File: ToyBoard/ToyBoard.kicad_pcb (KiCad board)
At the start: 2 copper layers, 41.3 x 41 mm, 18 parts, among them J5 MSD-1-A, Q1 NMOS, Q2 NMOS

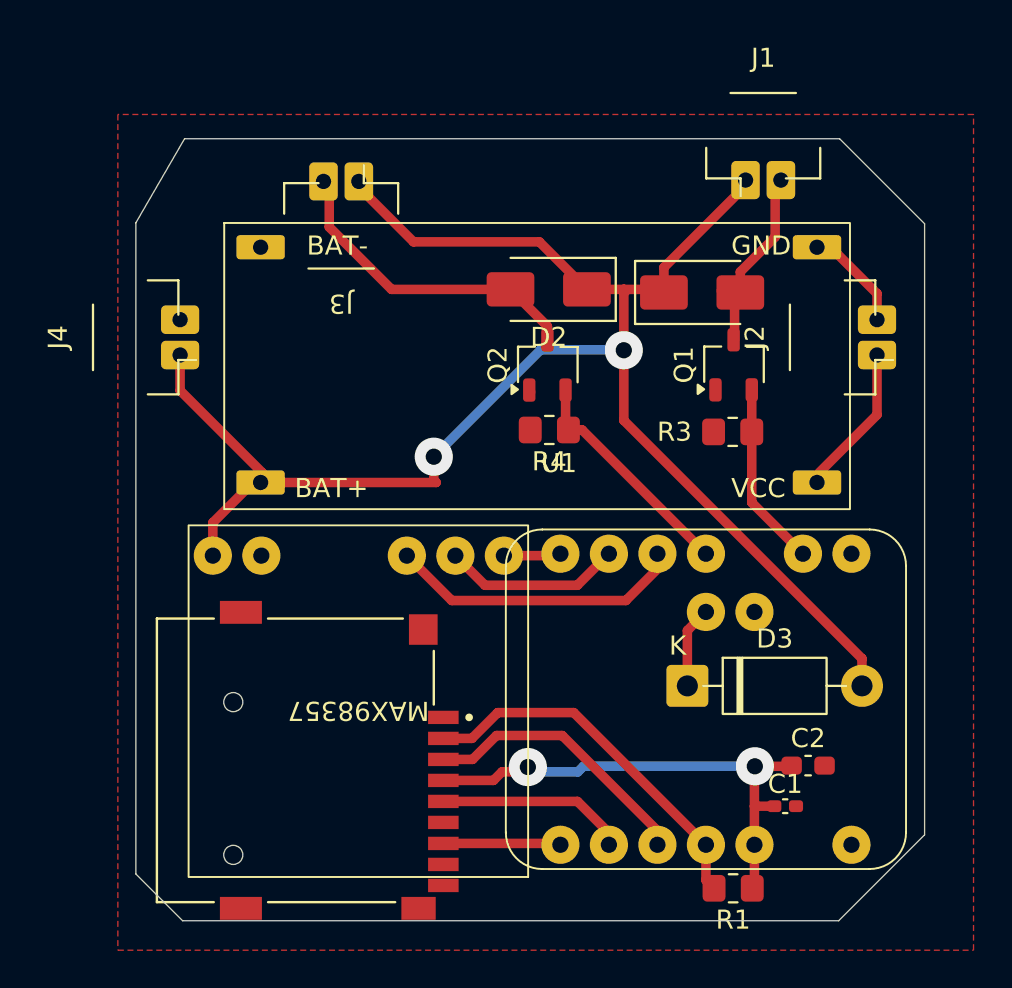
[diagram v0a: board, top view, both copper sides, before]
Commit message: Pcb and Gerbs for JLCPCB
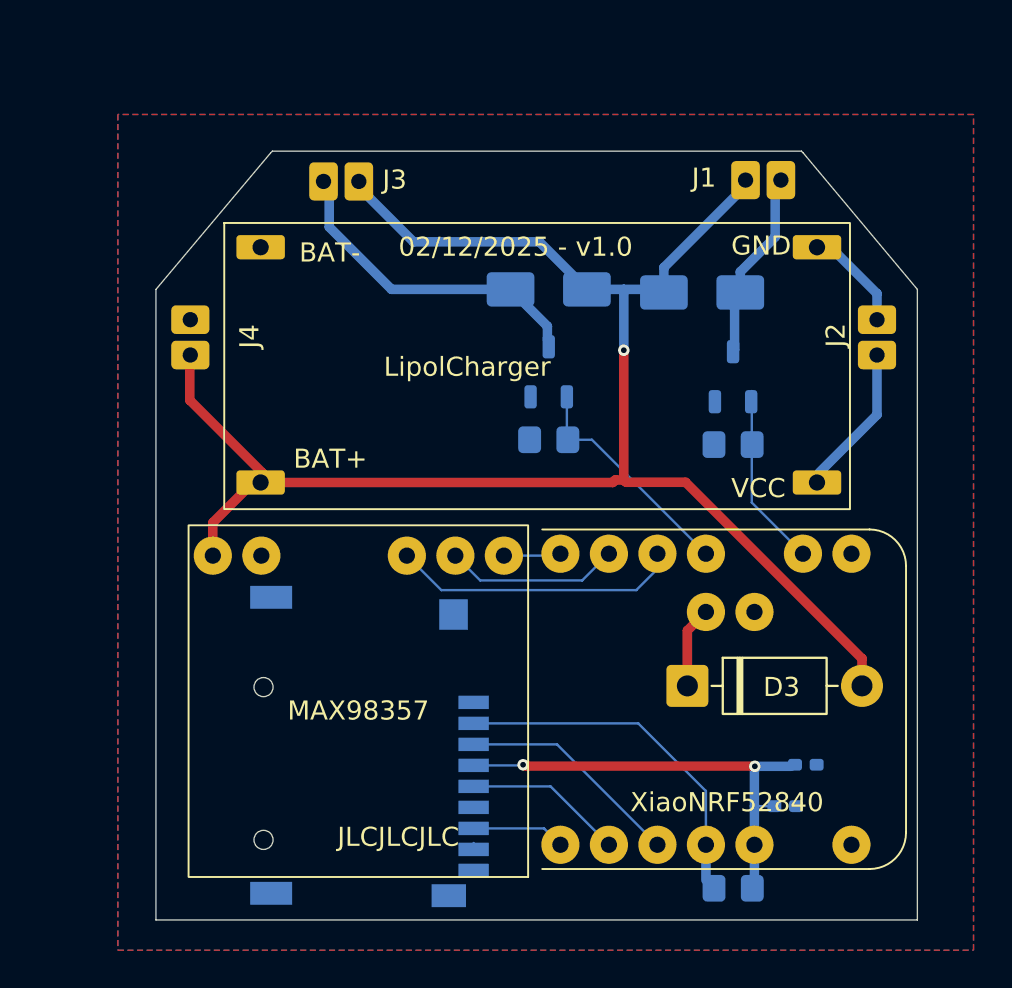
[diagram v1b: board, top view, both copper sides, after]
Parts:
- C1, D1, D2, J5, Q1, Q2, R1, R3, R4: moved to B.Cu
- C2: footprint Capacitor_SMD:C_0603_1608Metric_Pad1.08x0.95mm_HandSolder -> Capacitor_SMD:C_0402_1005Metric_Pad0.74x0.62mm_HandSolder; moved to B.Cu
- moved J5 1.77 mm to (126.0, 124.7), turned to 90 degrees
- moved R3 0.67 mm to (147.3, 109.0)
- moved Q1 0.62 mm to (147.3, 105.4)
- moved J4 0.54 mm to (117.6, 103.3)
- moved R4 0.51 mm to (137.7, 108.7)
- moved Q2 0.36 mm to (137.7, 105.2)
- moved C2 0.13 mm to (151.1, 125.7)
- renumbered U1 to LipolCharger, XiaoNRF1 to XiaoNRF52840
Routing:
- net BAT+: track 89.0 -> 86.3 mm, vias 2 -> 1
- net Net-(J5-VDD): track 26.3 -> 24.0 mm
- net Net-(J5-CMD): track 14.5 -> 12.5 mm
- net Net-(J5-CD/DAT3): track 19.6 -> 18.3 mm
- net Net-(J5-DAT0): track 6.16 -> 5.00 mm
- net Net-(J5-CLK): track 10.3 -> 9.28 mm
- added copper zone on B.Cu, net GND
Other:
- board size 41.3 x 41 mm -> 39.9 x 40.3 mm
- copper layers 2 -> 4
- board text added: "02/12/2025 - v1.0"
- board text added: "JLCJLCJLC"
- board text removed: "${REFERENCE}"
